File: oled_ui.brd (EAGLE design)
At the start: 84.5 x 19.2 mm, 42 parts, among them IC1 74HC14D

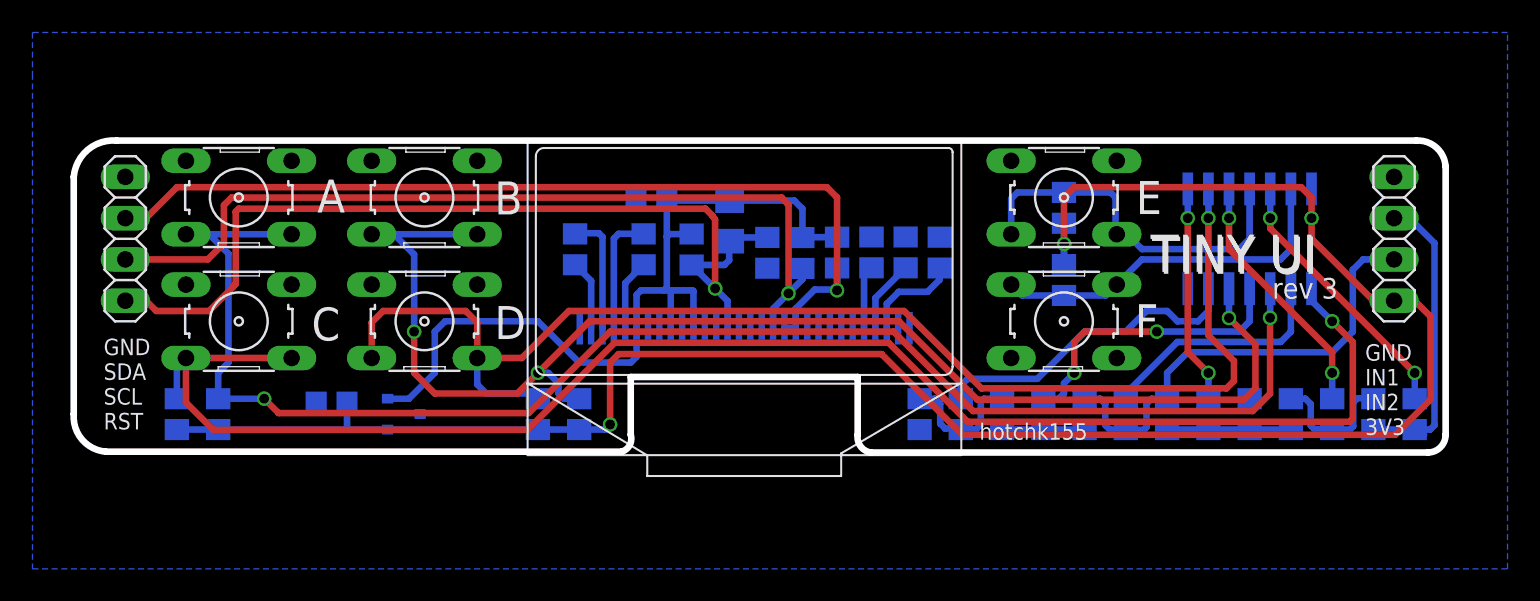
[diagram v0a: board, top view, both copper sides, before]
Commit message: ready?
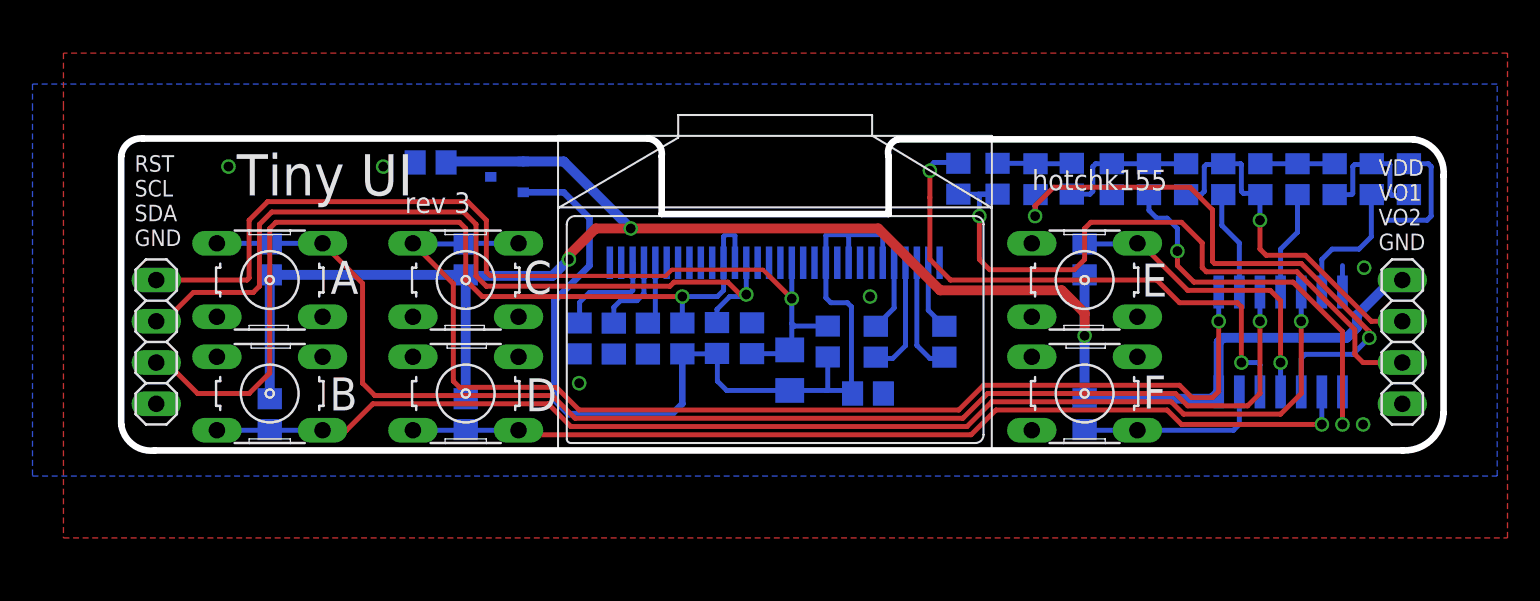
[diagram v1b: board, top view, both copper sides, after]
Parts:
- removed R11, R12, R13, R14, R15, R16, R17, R18, R19, R20, R21, R22, R23: (no value), rcl:R0805
- added 1A, 1B, 2A, 2B, 3A, 3B, 4A, 4B, 5B, 6B, 7B, 8B, J1: (no value), rcl:R0805
- moved U$1 44.1 mm to (56.5, 28.6), turned to 180 degrees
- moved C6 23.4 mm to (53.6, 8.90), turned to 270 degrees
- moved C3 22.8 mm to (31.1, 9.11), turned to 270 degrees
- moved R6 20.2 mm to (24.1, 14.0)
- moved R8 19.0 mm to (12.1, 4.45), turned to 90 degrees
- moved C4 18.7 mm to (33.2, 9.09), turned to 270 degrees
- moved C1 18.0 mm to (48.9, 5.71), turned to 180 degrees
- moved C2 16.1 mm to (22.0, 19.9)
- moved REG1 15.9 mm to (26.7, 19.1), turned to 270 degrees
- moved C5 15.4 mm to (49.4, 8.90), turned to 90 degrees
- moved B 15.4 mm to (12.1, 5.71)
- moved R1 14.8 mm to (35.3, 9.09), turned to 90 degrees
- moved C 14.2 mm to (24.1, 12.7), turned to 0 degrees
- moved R10 10.9 mm to (37.5, 9.11), turned to 90 degrees
- moved R2 10.1 mm to (46.4, 8.92), turned to 270 degrees
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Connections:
- net BUTTONS_OUT1: now also 4A.1, 8B.1; no longer R11.1, R17.1
- net BUTTONS_OUT2: now also 2A.1, 4B.1, J1.2; no longer R14.1, R20.2, R21.1
- net GND: now also 1B.2, 5B.2; no longer R19.2, R23.2
- net N$15: now also 3B.2; no longer R15.2
- net N$16: now also 2B.2; no longer R16.2
- net N$17: now also 1A.2, 1B.1, 2B.1; no longer R16.1, R22.2, R23.1
- net N$18: now also 1A.1, 2A.2, 3B.1; no longer R15.1, R21.2, R22.1
- net N$20: now also 6B.2; no longer R13.2
- net N$21: now also 3A.2, 5B.1, 6B.1, J1.1; no longer R13.1, R18.2, R19.1, R20.1
- net N$22: now also 7B.2; no longer R12.2
- net N$23: now also 3A.1, 4A.2, 7B.1; no longer R12.1, R17.2, R18.1
- net N$24: now also 8B.2; no longer R11.2
- net N$7: now also 4B.2; no longer R14.2
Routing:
- net N$11: track 97.9 -> 71.1 mm
- net BUTTONS_OUT1: track 19.0 -> 41.6 mm, vias 0 -> 1
- net N$12: track 79.6 -> 59.1 mm
- net N$22: track 15.5 -> 35.7 mm
- net N$24: track 16.6 -> 34.3 mm
- net N$9: track 94.9 -> 79.8 mm, vias 2 -> 1
- net N$15: track 18.2 -> 6.43 mm, vias 2 -> 0
- net N$16: track 19.8 -> 8.24 mm
- net N$20: track 13.4 -> 25.0 mm
- net 5V: track 127.1 -> 115.9 mm
- net N$14: track 22.4 -> 11.7 mm
- net 3V3: track 52.0 -> 61.0 mm
- net GND: track 0.00 -> 8.89 mm, vias 0 -> 6
- net N$7: track 14.7 -> 6.48 mm
- net N$5: track 83.8 -> 75.8 mm, vias 3 -> 1
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- added copper zone on layer 1, net GND
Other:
- board size 84.5 x 19.2 mm -> 81.4 x 19.2 mm
- board text added: "RST SCL SDA GND"
- board text added: "Tiny UI"
- board text added: "VDD VO1 VO2 GND"
- board text removed: "GND IN1 IN2 3V3"
- board text removed: "GND SDA SCL RST"
- board text removed: "TINY UI"
